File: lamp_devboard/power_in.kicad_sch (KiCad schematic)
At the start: 38 parts, among them J201 Screw_Terminal_01x02, J202 USB_C_Receptacle_USB2.0, J203 Conn_01x03, U201 TPS212x, U202 BQ24200, U203 FUSB302B01MPX, U204 TLV71318PDBV, U205 TLV71318PDBV

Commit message: some changes
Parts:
- removed JP203, JP205: Jumper_3_Open, Jumper:SolderJumper-3_P1.3mm_Open_RoundedPad1.0x1.5mm, symbol Jumper:Jumper_3_Open
- removed TP202, TP203, TP204, TP205: TestPoint, TestPoint:TestPoint_Pad_1.0x1.0mm, symbol Connector:TestPoint
- added D203: SM6T12A, Diode_SMD:D_SMB, symbol Diode:SM6T12A
- added F201: Fuse, Fuse:Fuse_1206_3216Metric_Pad1.42x1.75mm_HandSolder, symbol Device:Fuse
- added U207: USBLC6-4SC6, Package_TO_SOT_SMD:SOT-23-6, symbol Power_Protection:USBLC6-4SC6
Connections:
- net BatP: now also R201.1, R203.1, U201.7 (IN1); no longer R205.1, U201.2 (IN2)
- net GND: now also D203.2 (A2), U207.2 (GND)
- net Pout_: now also U204.3 (EN), U205.3 (EN)
- net TerminalPIn: now also R205.1, U201.2 (IN2), D203.1 (A1), F201.2; no longer J201.2 (Pin_2), R201.1, R203.1, U201.7 (IN1)
- net USB_DATA.D+: now also U207.6 (I/O4)
- net USB_DATA.D-: now also U207.4 (I/O3)
- net UsbPIn: now also U207.5 (VBUS)
- net at J202.A5 (CC1), R209.1: now also U207.3 (I/O2)
- net at J202.B5 (CC2), R208.1: now also U207.1 (I/O1)
- new net TerminalPIn_: F201.1, J201.2 (Pin_2)
- no-connect marks 0 -> 4
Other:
- moved on the sheet: C201, C202, C203, C204, C205, C206, C207, C208, D201, D202, J201, J202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

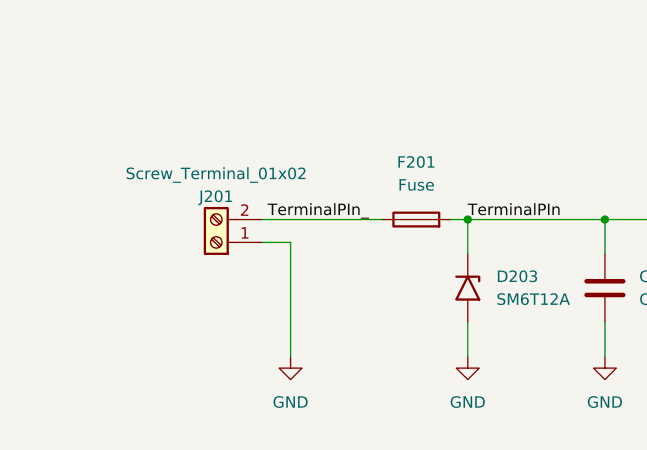
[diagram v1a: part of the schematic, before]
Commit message: some small changes
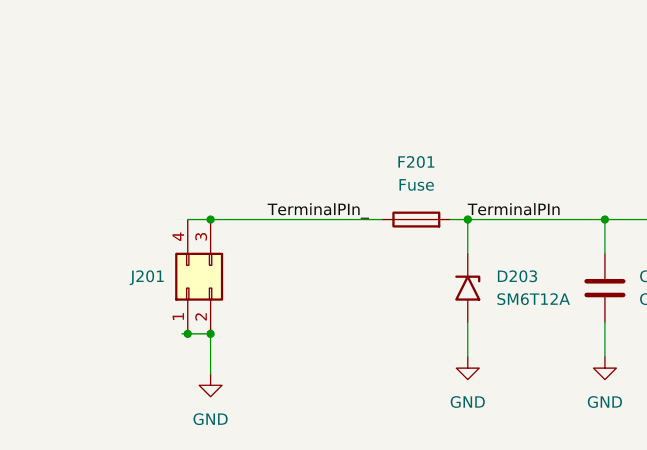
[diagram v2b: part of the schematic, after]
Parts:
- removed J201: Screw_Terminal_01x02, TerminalBlock:TerminalBlock_bornier-2_P5.08mm, symbol Connector:Screw_Terminal_01x02
- added J201: Conn_02x02_Counter_Clockwise, Connector_PinSocket_2.54mm:PinSocket_2x02_P2.54mm_Vertical, symbol Connector_Generic:Conn_02x02_Counter_Clockwise
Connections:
- net GND: now also J201.1 (Pin_1), J201.2 (Pin_2)
- net TerminalPIn_: now also J201.3 (Pin_3), J201.4 (Pin_4)
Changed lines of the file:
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@@
 (kicad_sch (version 20211123) (generator eeschema)
   (paper "A3")
+  (junction (at 45.085 212.09) (diameter 0) (color 0 0 0 0)
+  )
   (junction (at 336.55 78.105) (diameter 0) (color 0 0 0 0)
   )
+  (junction (at 45.085 199.39) (diameter 0) (color 0 0 0 0)
+  )
   (junction (at 336.55 111.125) (diameter 0) (color 0 0 0 0)
   )
@@
   )
   (junction (at 77.47 38.735) (diameter 0) (color 0 0 0 0)
+  )
+  (junction (at 42.545 212.09) (diameter 0) (color 0 0 0 0)
   )
   (junction (at 73.66 199.39) (diameter 0) (color 0 0 0 0)
@@
     (stroke (width 0) (type default) (color 0 0 0 0))
   )
-  (wire (pts (xy 50.8 201.93) (xy 53.975 201.93))
+  (wire (pts (xy 41.91 212.09) (xy 42.545 212.09))
     (stroke (width 0) (type default) (color 0 0 0 0))
   )
@@
     (stroke (width 0) (type default) (color 0 0 0 0))
   )
-  (wire (pts (xy 53.975 201.93) (xy 53.975 214.63))
+  (wire (pts (xy 45.085 212.09) (xy 45.085 216.535))
     (stroke (width 0) (type default) (color 0 0 0 0))
   )
@@
     (stroke (width 0) (type default) (color 0 0 0 0))
   )
+  (wire (pts (xy 42.545 212.09) (xy 45.085 212.09))
+    (stroke (width 0) (type default) (color 0 0 0 0))
+  )
   (wire (pts (xy 264.16 78.105) (xy 272.415 78.105))
     (stroke (width 0) (type default) (color 0 0 0 0))
@@
     (stroke (width 0) (type default) (color 0 0 0 0))
   )
+  (wire (pts (xy 45.085 199.39) (xy 64.135 199.39))
+    (stroke (width 0) (type default) (color 0 0 0 0))
+  )
   (bus (pts (xy 116.84 137.16) (xy 125.095 137.16))
     (stroke (width 0) (type default) (color 0 0 0 0))
@@
     (stroke (width 0) (type default) (color 0 0 0 0))
   )
-  (wire (pts (xy 64.135 199.39) (xy 50.8 199.39))
+  (wire (pts (xy 42.545 199.39) (xy 45.085 199.39))
     (stroke (width 0) (type default) (color 0 0 0 0))
   )
@@
     (pin "2")
   )
-  (symbol (lib_id "power:GND") (at 53.975 214.63 0) (unit 1)
-    (in_bom yes) (on_board yes) (fields_autoplaced)
-    (property "Reference" "#PWR0107" (id 0) (at 53.975 220.98 0)
-      (effects (font (size 1.27 1.27)) hide)
-    )
-    (property "Value" "GND" (id 1) (at 53.975 219.71 0))
-    (property "Footprint" "" (id 2) (at 53.975 214.63 0)
-      (effects (font (size 1.27 1.27)) hide)
-    )
-    (property "Datasheet" "" (id 3) (at 53.975 214.63 0)
+  (symbol (lib_id "power:GND") (at 45.085 216.535 0) (unit 1)
+    (in_bom yes) (on_board yes) (fields_autoplaced)
+    (property "Reference" "#PWR0107" (id 0) (at 45.085 222.885 0)
+      (effects (font (size 1.27 1.27)) hide)
+    )
+    (property "Value" "GND" (id 1) (at 45.085 221.615 0))
+    (property "Footprint" "" (id 2) (at 45.085 216.535 0)
+      (effects (font (size 1.27 1.27)) hide)
+    )
+    (property "Datasheet" "" (id 3) (at 45.085 216.535 0)
       (effects (font (size 1.27 1.27)) hide)
     )
@@
     )
     (pin "1")
-  )
-  (symbol (lib_id "Connector:Screw_Terminal_01x02") (at 45.72 201.93 180) (unit 1)
-    (in_bom yes) (on_board yes)
-    (property "Reference" "J201" (id 0) (at 45.72 196.85 0))
-    (property "Value" "Screw_Terminal_01x02" (id 1) (at 45.72 194.31 0))
-    (property "Footprint" "TerminalBlock:TerminalBlock_bornier-2_P5.08mm" (id 2) (at 46.355 198.12 0)
-      (effects (font (size 1.27 1.27)) hide)
-    )
-    (property "Datasheet" "~" (id 3) (at 45.72 201.93 0)
-      (effects (font (size 1.27 1.27)) hide)
-    )
-    (pin "1")
-    (pin "2")
   )
   (symbol (lib_id "Device:R") (at 266.7 119.38 0) (unit 1)
@@
     (pin "1")
   )
+  (symbol (lib_id "Connector_Generic:Conn_02x02_Counter_Clockwise") (at 42.545 207.01 90) (unit 1)
+    (in_bom yes) (on_board yes)
+    (property "Reference" "J201" (id 0) (at 36.195 205.74 90)
+      (effects (font (size 1.27 1.27)) (justify right))
+    )
+    (property "Value" "Conn_02x02_Counter_Clockwise" (id 1) (at 47.625 207.0099 90)
+      (effects (font (size 1.27 1.27)) (justify right) hide)
+    )
+    (property "Footprint" "Connector_PinSocket_2.54mm:PinSocket_2x02_P2.54mm_Vertical" (id 2) (at 42.545 207.01 0)
+      (effects (font (size 1.27 1.27)) hide)
+    )
+    (property "Datasheet" "~" (id 3) (at 42.545 207.01 0)
+      (effects (font (size 1.27 1.27)) hide)
+    )
+    (pin "1")
+    (pin "2")
+    (pin "3")
+    (pin "4")
+  )
 )
